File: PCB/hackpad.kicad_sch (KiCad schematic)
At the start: 34 parts, among them SW11 SW_Push, SW12 SW_Push, SW13 SW_Push, SW14 SW_Push, SW15 SW_Push, SW16 SW_Push, SW17 SW_Push, SW18 SW_Push, SW19 SW_Push, SW4 RotaryEncoder_Switch, U1 MOUDLE-SEEEDUINO-XIAO, U2 ER_OLEDM0.91_1x-I2C

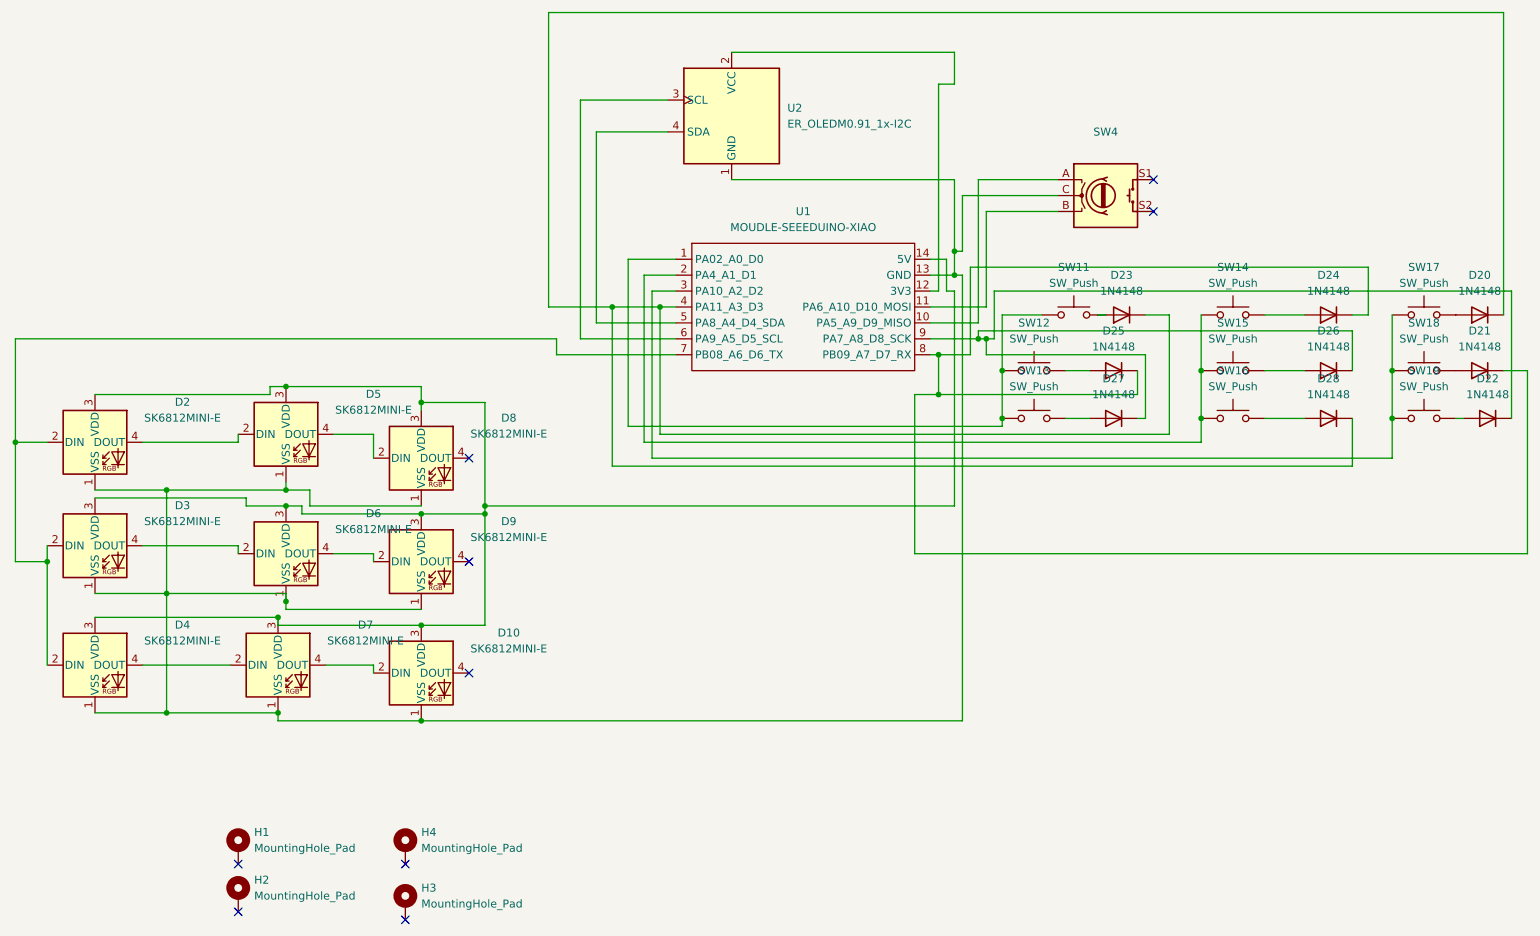
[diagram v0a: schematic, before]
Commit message: Add files via upload
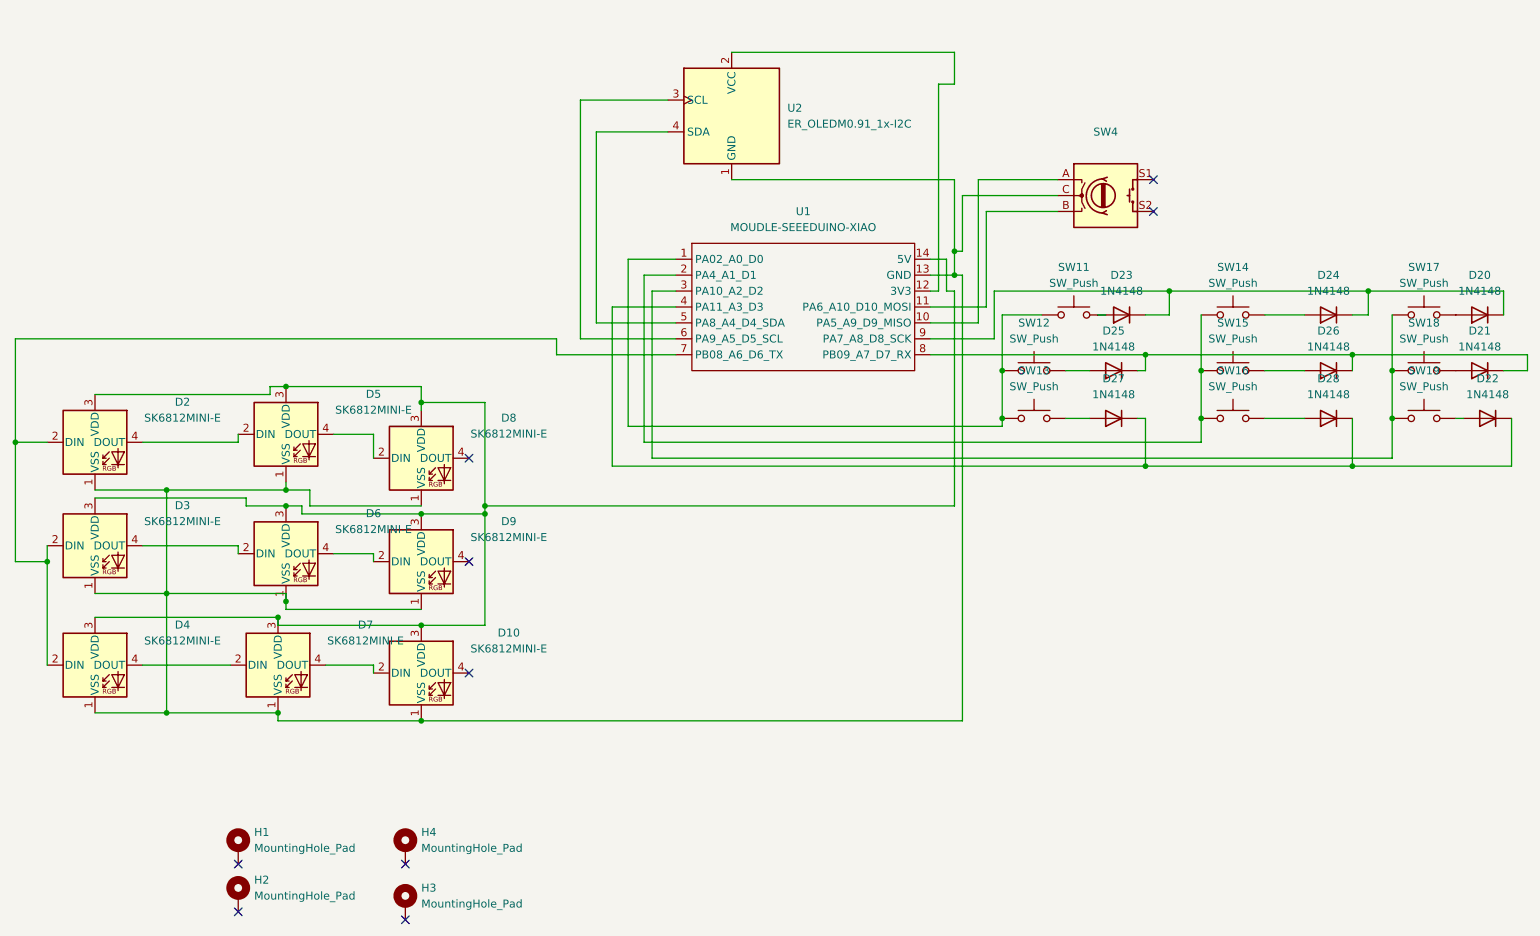
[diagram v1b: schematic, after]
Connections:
- net at D21.1 (K), D25.1 (K), U1.8 (PB09_A7_D7_RX): now also D26.1 (K); no longer D24.1 (K)
- net at D20.1 (K), D23.1 (K): now also D24.1 (K), U1.9 (PA7_A8_D8_SCK); no longer D28.1 (K), U1.4 (PA11_A3_D3)
- net at D22.1 (K), D27.1 (K): now also D28.1 (K), U1.4 (PA11_A3_D3); no longer D26.1 (K), U1.9 (PA7_A8_D8_SCK)

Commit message: Add files via upload
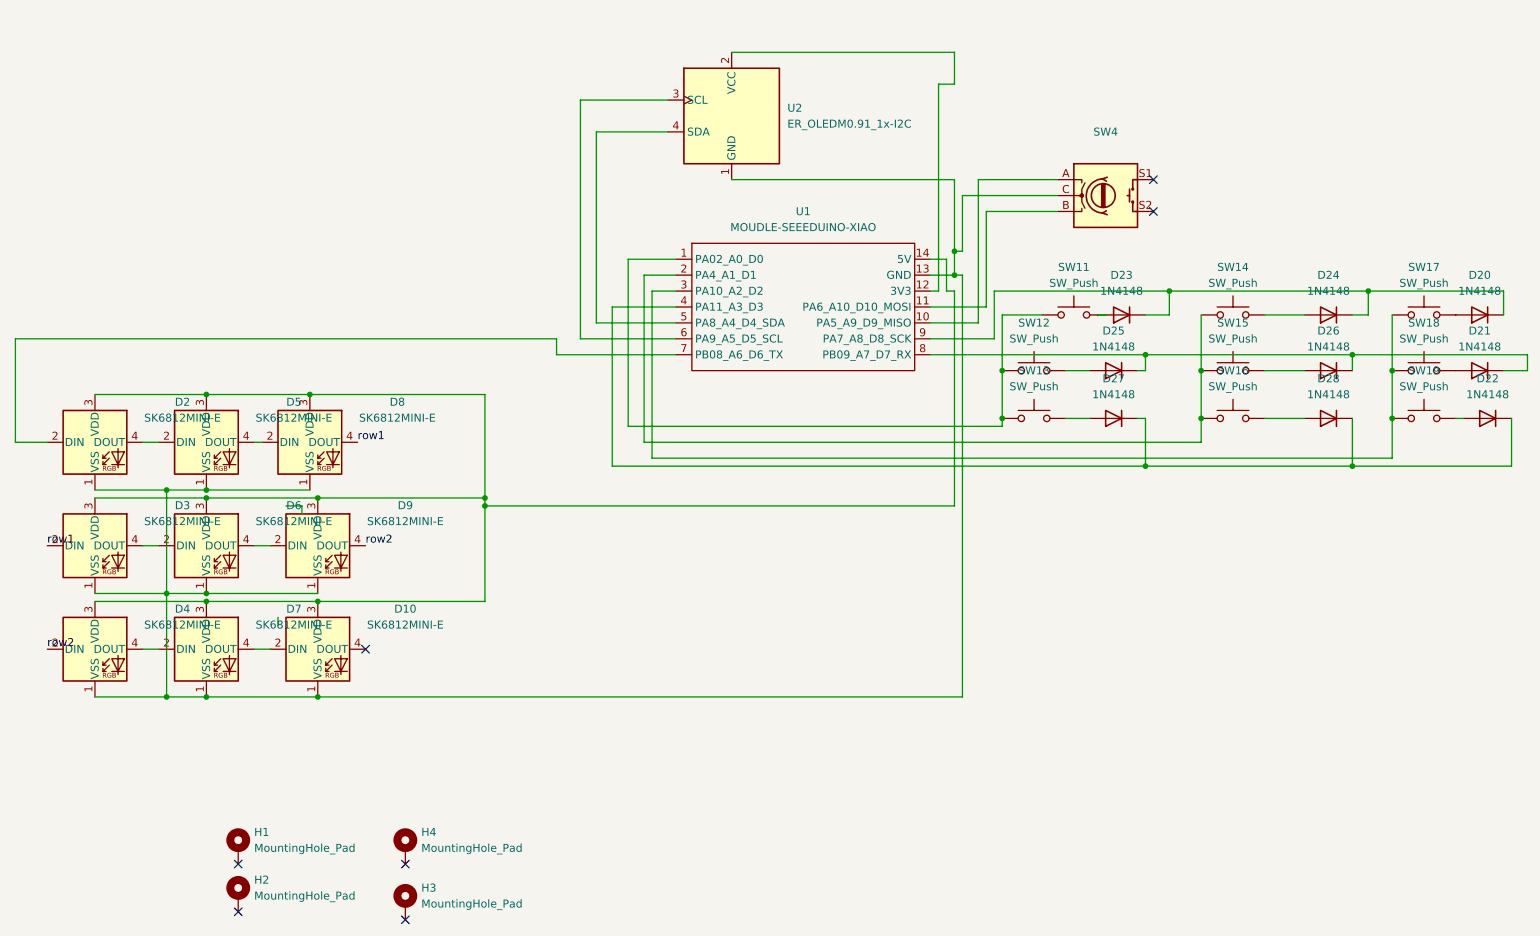
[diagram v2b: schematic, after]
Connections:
- net at D2.2 (DIN), U1.7 (PB08_A6_D6_TX): no longer D3.2 (DIN), D4.2 (DIN)
- net row2: now reaches D9.4 (DOUT)
- net row2: now also D4.2 (DIN)
- net row1: now reaches D8.4 (DOUT)
- net row1: now also D3.2 (DIN)
- no-connect marks 9 -> 7
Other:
- moved on the sheet: D10, D4, D5, D6, D7, D8, D9
